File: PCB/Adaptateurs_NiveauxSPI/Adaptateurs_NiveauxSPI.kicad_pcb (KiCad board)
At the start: 2 copper layers, 21 parts, among them P1 CONN_01X07, P2 CONN_01X08, P3 CONN_01X07, P4 CONN_01X12, P5 CONN_01X07, P6 CONN_01X09, P7 CONN_01X07, P8 CONN_01X10, U1 CON_5V_3-3V, U2 CON_5V_3-3V, U3 CON_5V_3-3V, U4 CON_5V_3-3V

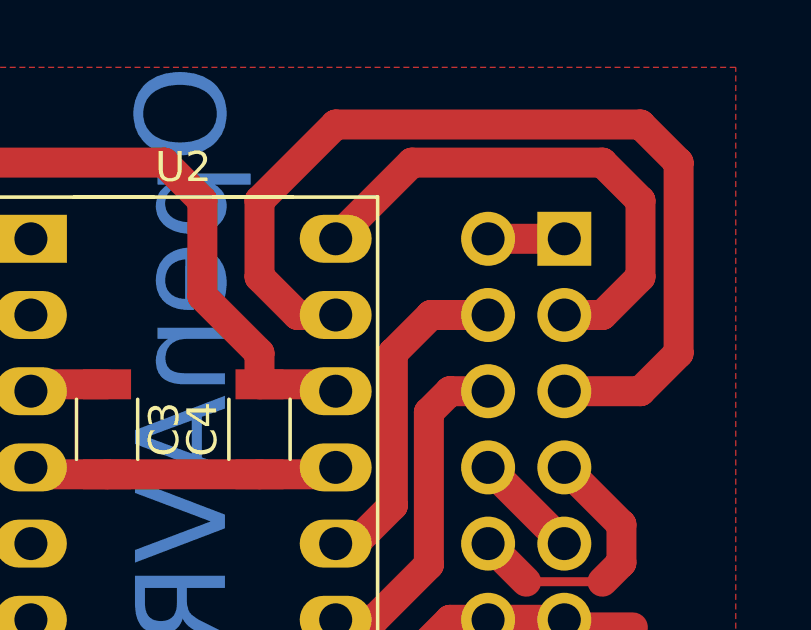
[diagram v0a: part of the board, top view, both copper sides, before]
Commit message: Fix merging changes
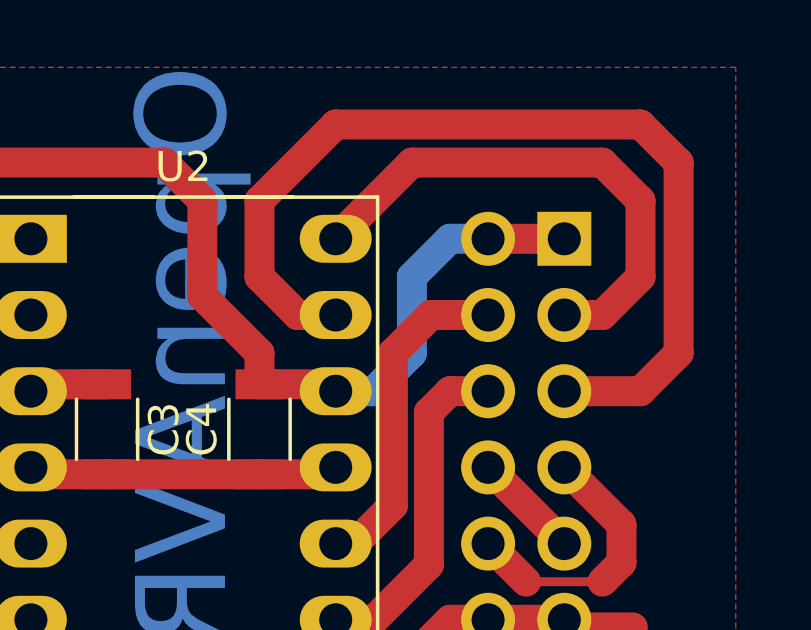
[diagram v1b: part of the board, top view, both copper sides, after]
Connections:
- P4 pad 1: Net-(P4-Pad1) -> +3.3V
- P4 pad 2: Net-(P4-Pad1) -> +3.3V
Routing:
- net +3.3V: track 20.9 -> 32.1 mm
- net Net-(P4-Pad1): track 2.54 -> 0.00 mm

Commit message: Merge from Ingwie/V3
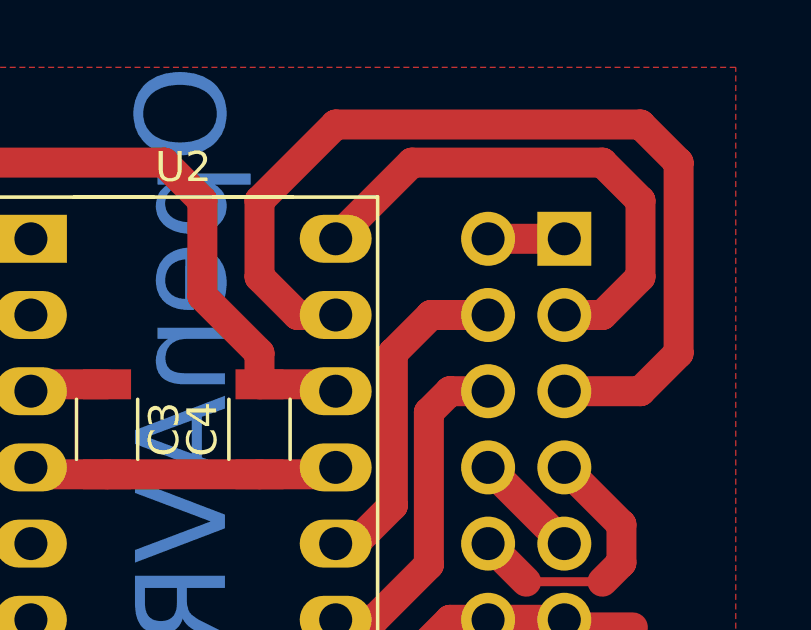
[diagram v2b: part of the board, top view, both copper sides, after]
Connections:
- P4 pad 1: +3.3V -> Net-(P4-Pad1)
- P4 pad 2: +3.3V -> Net-(P4-Pad1)
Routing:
- net +3.3V: track 32.1 -> 20.9 mm
- net Net-(P4-Pad1): track 0.00 -> 2.54 mm
